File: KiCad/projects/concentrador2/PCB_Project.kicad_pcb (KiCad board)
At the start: 2 copper layers, 91.4 x 88 mm, 43 parts, among them J1 54602-908LF, P1 Grabador, P2 Entrada fuente externa, P4 Header 20X2, P5 Header 2, U1 DSPIC33EP256MC202-I/SP, U2 STEP_DOWN_CONVERTER, U3 LD33V, U4 MAX485, U5 DS3234S#, U9 MAX485

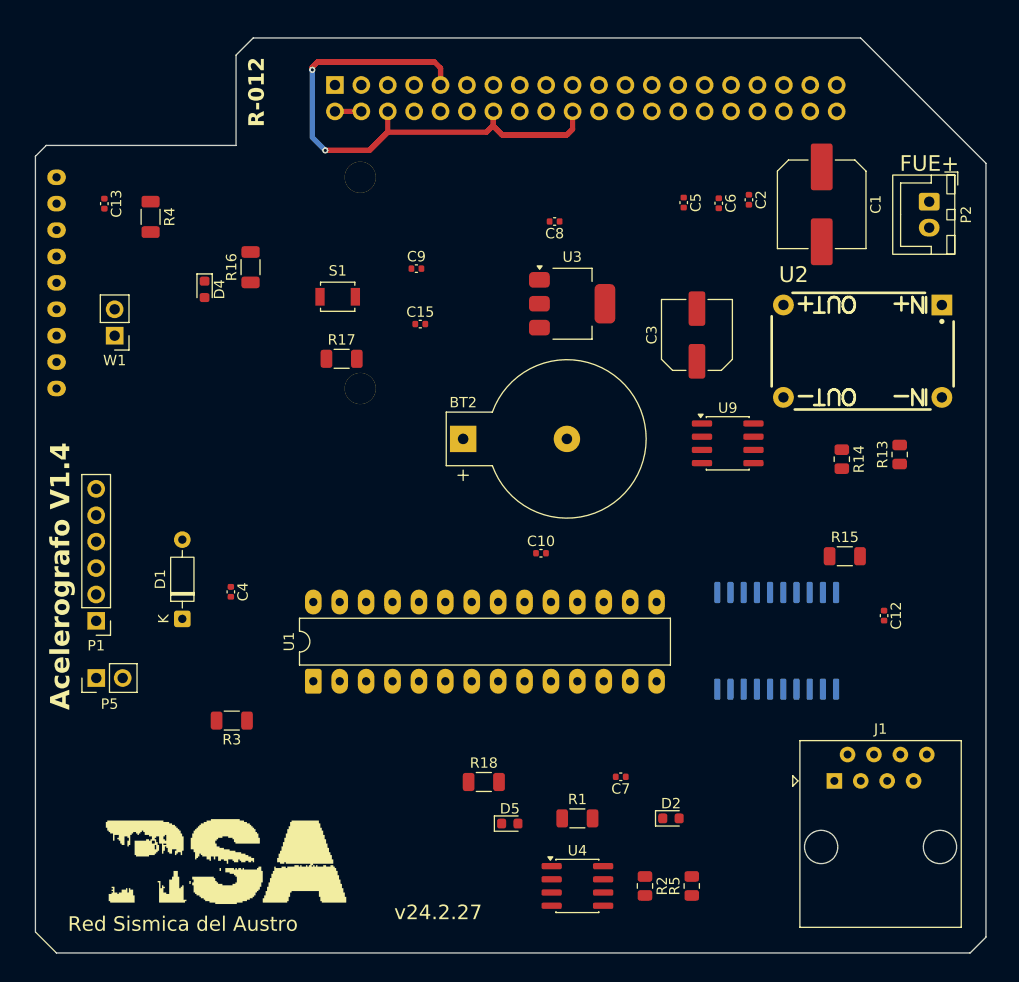
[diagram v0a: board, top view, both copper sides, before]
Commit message: Archivos Gerber
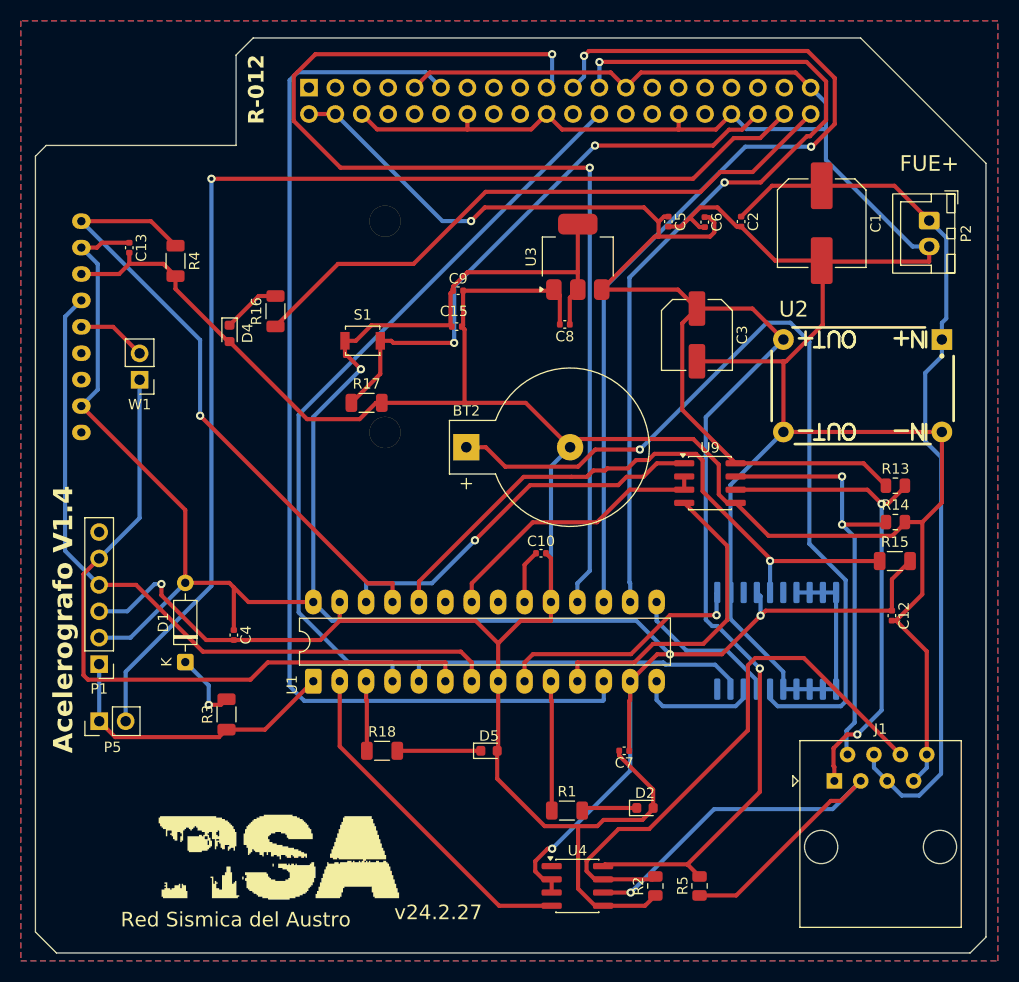
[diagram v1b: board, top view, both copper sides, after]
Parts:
- moved R18 10.2 mm to (136.1, 129.6)
- moved C8 9.95 mm to (153.7, 88.6)
- moved R14 7.95 mm to (185.5, 107.6), turned to 0 degrees
- moved D5 7.28 mm to (146.4, 129.6)
- moved C13 4.87 mm to (111.8, 81.2)
- moved R16 4.87 mm to (125.9, 87.3)
- moved D4 4.87 mm to (121.5, 89.4)
- moved R17 4.87 mm to (134.6, 96.1)
- moved R4 4.87 mm to (116.3, 82.4)
- moved S1 4.87 mm to (134.3, 90.1)
- moved W1 4.87 mm to (112.8, 93.9)
- moved GPS1 4.85 mm to (107.2, 78.6)
- moved R15 4.84 mm to (185.5, 111.3)
- moved U3 4.54 mm to (155.0, 82.1), turned to 90 degrees
- moved C9 4.54 mm to (143.4, 85.3)
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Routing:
- net GND: track 95.9 -> 517.5 mm, vias 2 -> 1
- net VCC: track 0.00 -> 239.7 mm, vias 0 -> 4
- net 5V: track 2.54 -> 177.9 mm, vias 0 -> 2
- net RESET: track 0.00 -> 113.3 mm, vias 0 -> 1
- net SPI1_MOSI: track 0.00 -> 106.1 mm, vias 0 -> 2
- net RPI_INT1: track 0.38 -> 106.4 mm
- net SPI1_MISO: track 0.00 -> 92.2 mm, vias 0 -> 2
- net FUENTE_12V: track 0.00 -> 85.8 mm
- net SPI1_SCK: track 0.00 -> 85.2 mm, vias 0 -> 2
- net NetBT1_0: track 0.00 -> 85.0 mm, vias 0 -> 1
- net SPI1_DSPIC_SS: track 0.00 -> 72.8 mm
- net DSPIC_TX: track 0.00 -> 70.1 mm
- net _DSPIC_RX: track 0.00 -> 68.1 mm
- net DS3231_SQW: track 0.00 -> 60.6 mm, vias 0 -> 1
- net GPS_1PPS: track 0.00 -> 60.5 mm, vias 0 -> 1
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- added copper zone on B.Cu, net GND
- added copper zone on F.Cu, net GND
